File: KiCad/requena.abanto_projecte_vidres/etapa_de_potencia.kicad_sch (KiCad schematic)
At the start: 15 parts, among them U1 L298N, U2 TSR2-2450, U3 MCP6022, U4 LM1117DT-3.3

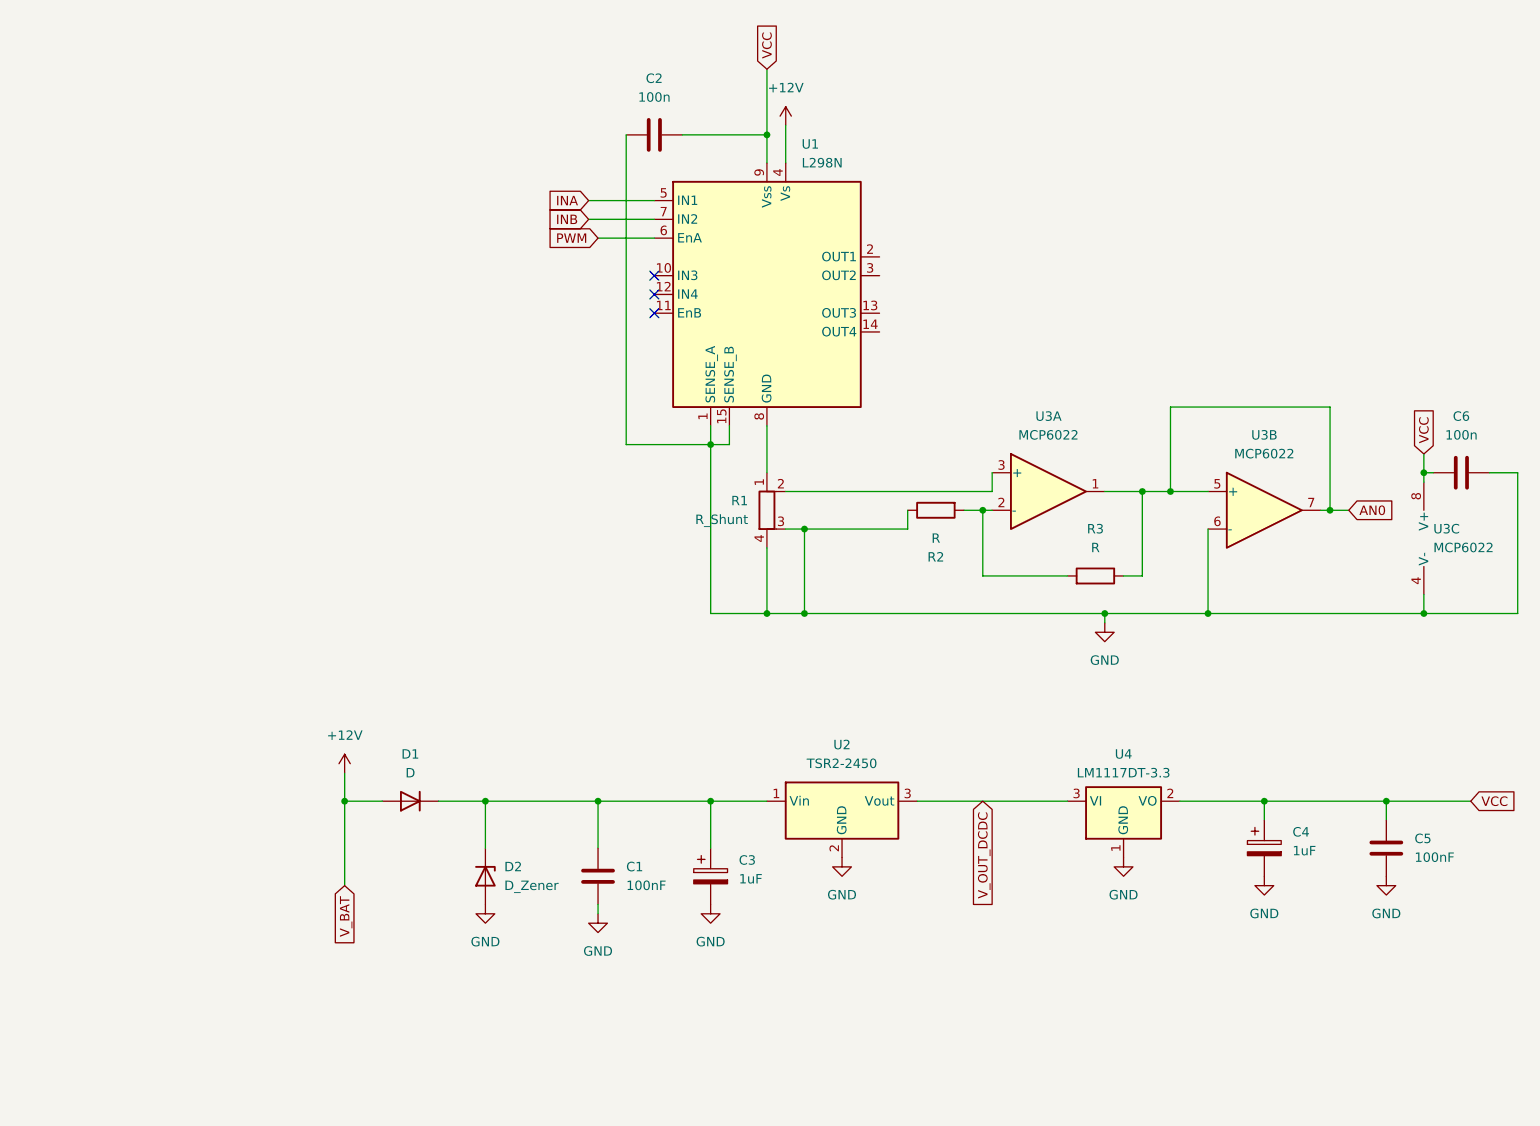
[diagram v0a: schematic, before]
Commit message: millora_petjades
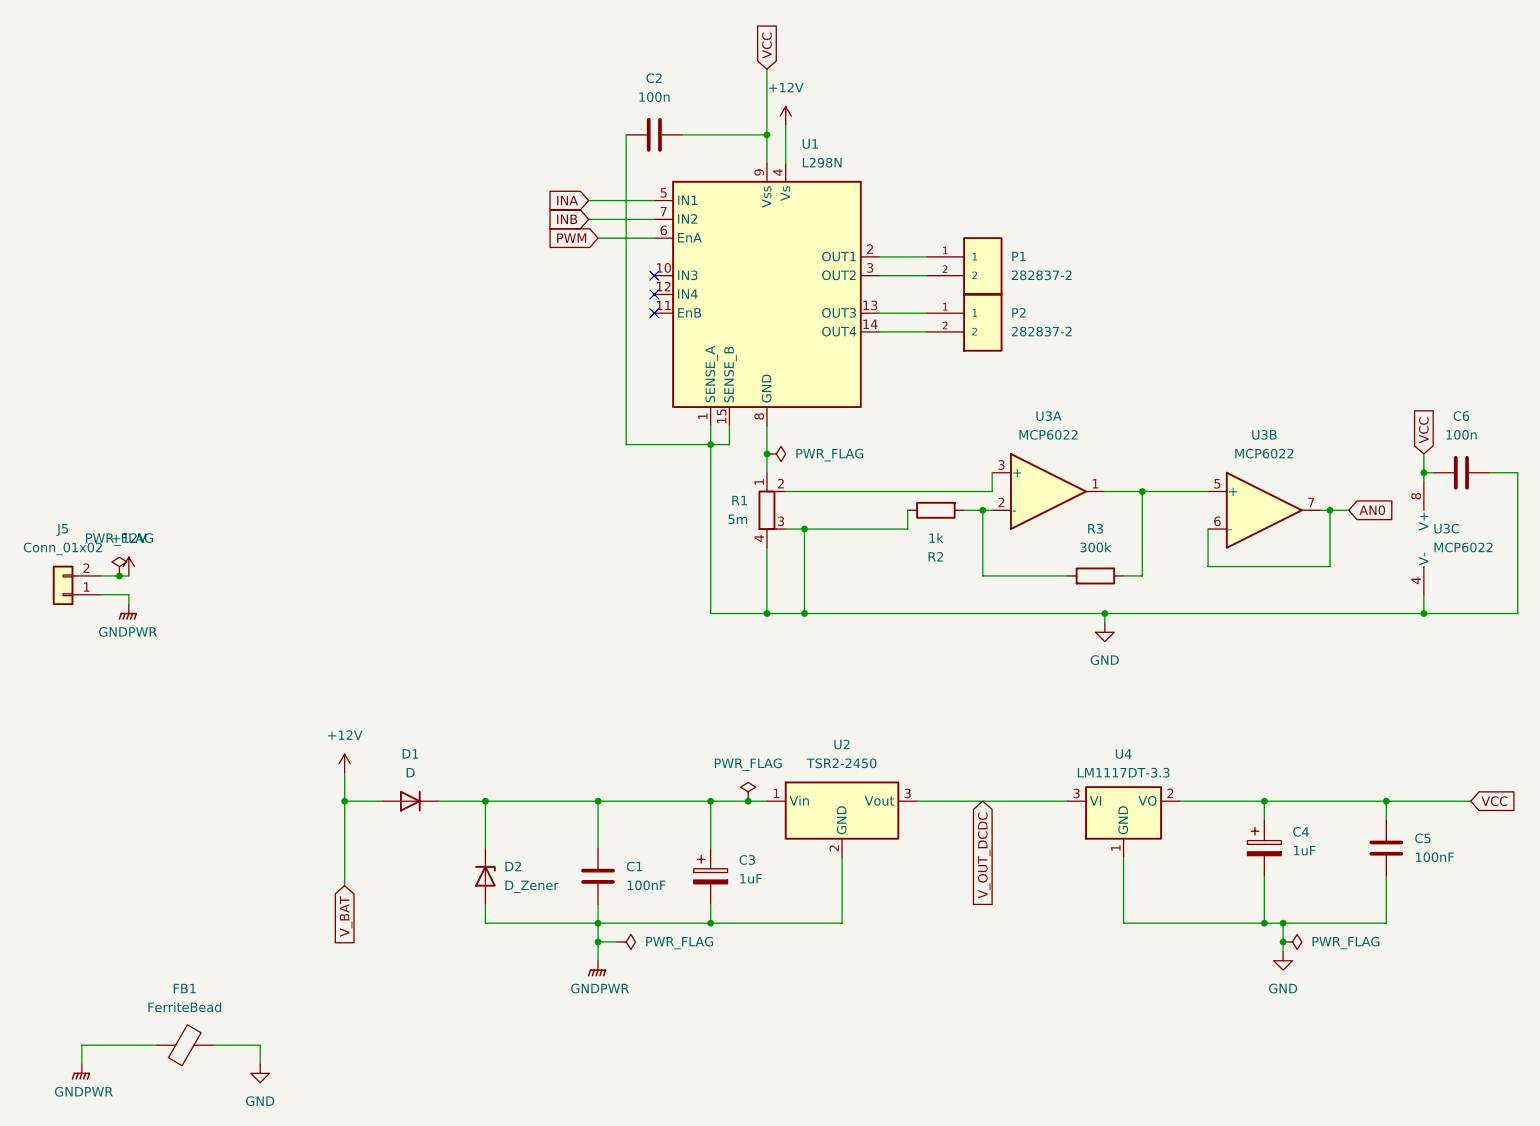
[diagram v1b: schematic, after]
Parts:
- added FB1: FerriteBead, Inductor_SMD:L_0805_2012Metric, symbol Device:FerriteBead
- added J5: Conn_01x02, TerminalBlock:TerminalBlock_Xinya_XY308-2.54-2P_1x02_P2.54mm_Horizontal, symbol Connector_Generic:Conn_01x02
- added P1, P2: 282837-2, 282837-2:TE_282837-2, symbol 282837-2:282837-2
- C1, C5: footprint (none) -> Capacitor_SMD:C_0805_2012Metric
- C2, C6: footprint (none) -> Capacitor_SMD:C_1206_3216Metric
- C3, C4: footprint (none) -> Capacitor_THT:CP_Radial_D4.0mm_P1.50mm
- D1: footprint (none) -> Diode_THT:D_DO-41_SOD81_P12.70mm_Horizontal
- D2: footprint (none) -> Diode_THT:D_A-405_P2.54mm_Vertical_AnodeUp
- R1: value R_Shunt -> 5m; footprint (none) -> Resistor_SMD:R_1206_3216Metric
- R2: value R -> 1k; footprint (none) -> Resistor_SMD:R_1206_3216Metric
- R3: value R -> 300k; footprint (none) -> Resistor_SMD:R_1206_3216Metric
- U3: footprint (none) -> Package_SO:SOIC-8_3.9x4.9mm_P1.27mm
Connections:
- net +12V: now also J5.2 (Pin_2)
- net AN0: now also U3.6 (-); no longer R3.1, U3.1, U3.5 (+)
- net GND: now also FB1.2; no longer C1.2, C3.2, D2.2 (A), U2.2 (GND), U3.6 (-)
- net at U1.13 (OUT3): now also P2.1
- net at U1.14 (OUT4): now also P2.2
- net at U1.2 (OUT1): now also P1.1
- net at U1.3 (OUT2): now also P1.2
- new net: R3.1, U3.1, U3.5 (+)
- new net GNDPWR: C1.2, C3.2, D2.2 (A), FB1.1, J5.1 (Pin_1), U2.2 (GND)

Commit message: milora_esquema_i_layoutcomençat
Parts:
- P1, P2: footprint 282837-2:TE_282837-2 -> motor_connector:TE_282837-2
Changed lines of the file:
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@@
 			)
 		)
-		(property "Footprint" "282837-2:TE_282837-2"
+		(property "Footprint" "motor_connector:TE_282837-2"
 			(at 148.59 53.34 0)
 			(effects
@@
 			)
 		)
-		(property "Footprint" "282837-2:TE_282837-2"
+		(property "Footprint" "motor_connector:TE_282837-2"
 			(at 148.59 60.96 0)
 			(effects
